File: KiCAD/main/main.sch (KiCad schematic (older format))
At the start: 6 parts, among them IC1 DHT22, J1 Charge Controller, J2 Sound Sensor, J3 BuckConverter, J4 Anemometer

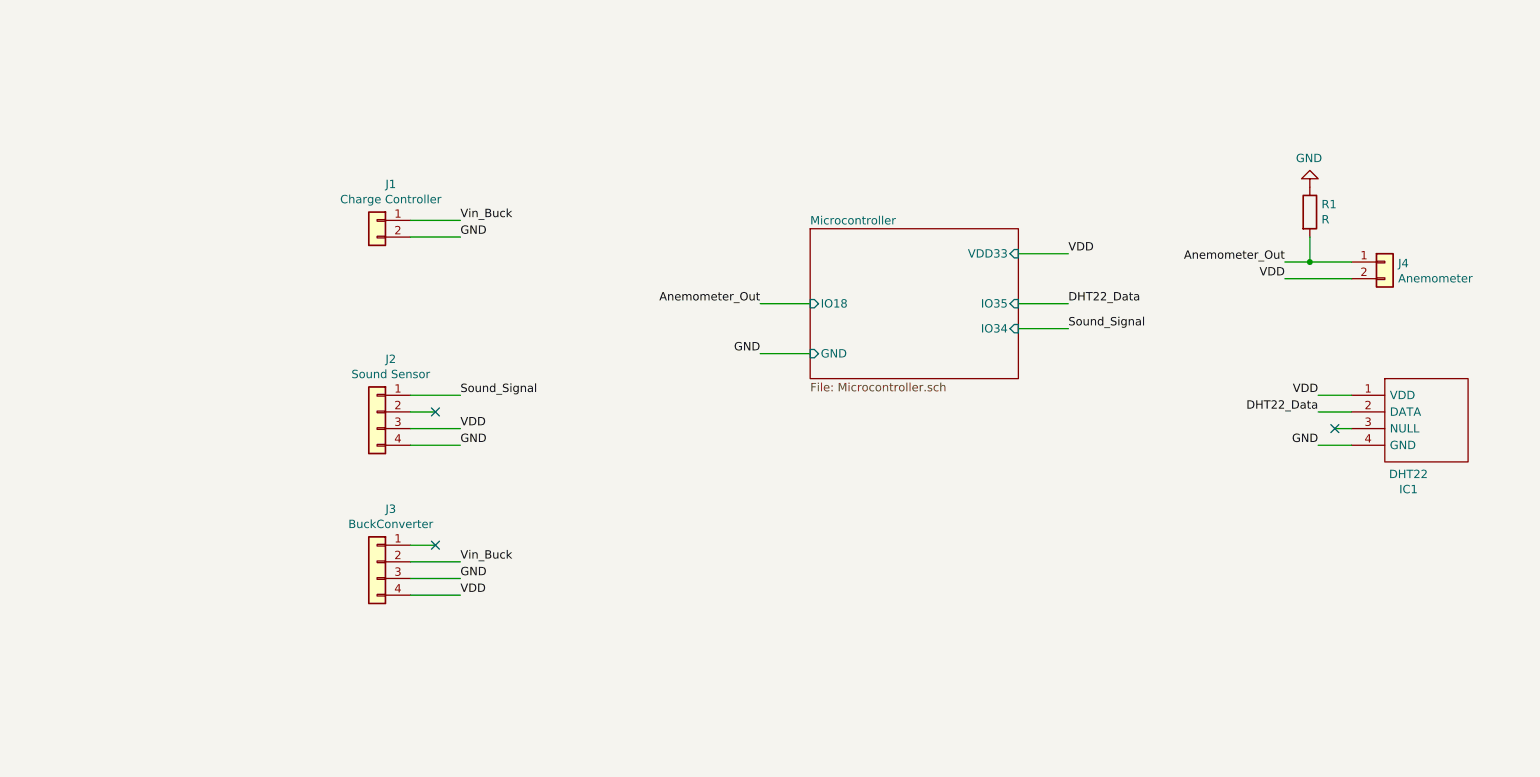
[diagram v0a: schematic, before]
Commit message: alimentação e proteção
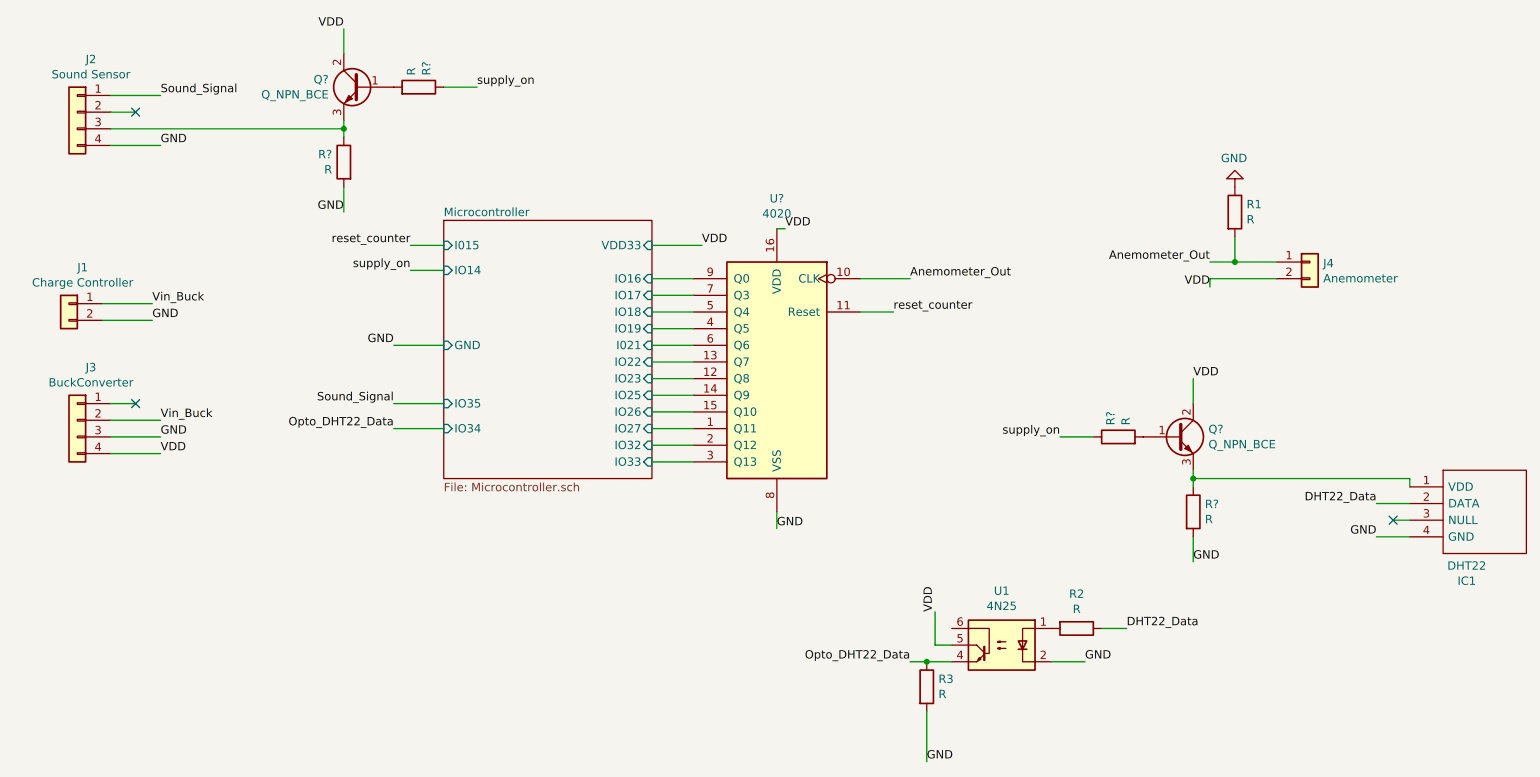
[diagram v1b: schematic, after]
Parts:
- added Q? (x2): Q_NPN_BCE, symbol Device:Q_NPN_BCE
- added R2: R, symbol Device:R
- added R3, R? (x4): R, Resistor_SMD:R_1206_3216Metric, symbol Device:R
- added U1: 4N25, Package_DIP:DIP-6_W7.62mm, symbol Isolator:4N25
- added U?: 4020, symbol 4xxx:4020
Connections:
- net Anemometer_Out: now also U?.10 (CLK)
- net DHT22_Data: now also R2.1
- net GND: now also R3.2, R?.2, R?.2, U1.2, U?.8 (VSS)
- net VDD: now also Q?.2 (C), Q?.2 (C), U1.5, U?.16 (VDD); no longer IC1.1 (VDD), J2.3 (Pin_3)
- new net: IC1.1 (VDD), Q?.3 (E), R?.1
- new net: J2.3 (Pin_3), Q?.3 (E), R?.1
- new net: R2.2, U1.1
- new net: Q?.1 (B), R?.2 (x2)
- new net Microcontroller/I021: U?.6 (Q6)
- new net Microcontroller/IO16: U?.9 (Q0)
- new net Microcontroller/IO17: U?.7 (Q3)
- new net Microcontroller/IO18: U?.5 (Q4)
- new net Microcontroller/IO19: U?.4 (Q5)
- new net Microcontroller/IO22: U?.13 (Q7)
- new net Microcontroller/IO23: U?.12 (Q8)
- new net Microcontroller/IO25: U?.14 (Q9)
- new net Microcontroller/IO26: U?.15 (Q10)
- new net Microcontroller/IO27: U?.1 (Q11)
- new net Microcontroller/IO32: U?.2 (Q12)
- new net Microcontroller/IO33: U?.3 (Q13)
- new net Opto_DHT22_Data: R3.1, U1.4
- new net reset_counter: U?.11 (Reset)
- new net supply_on: R?.1, R?.1
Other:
- moved on the sheet: IC1, J1, J2, J3, J4, R1
